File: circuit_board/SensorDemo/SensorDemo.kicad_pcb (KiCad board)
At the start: 4 copper layers, 65 x 57.5 mm, 56 parts, among them K1 PB, P1 CONN3X2, P2 CONN3X2, U1 TLV1117-33CDCYR, U2 dsPIC33EP32GP502, U3 LTC1658, U4 INA126, U5 REF1925, U6 REF1925, X1 CRYSTAL

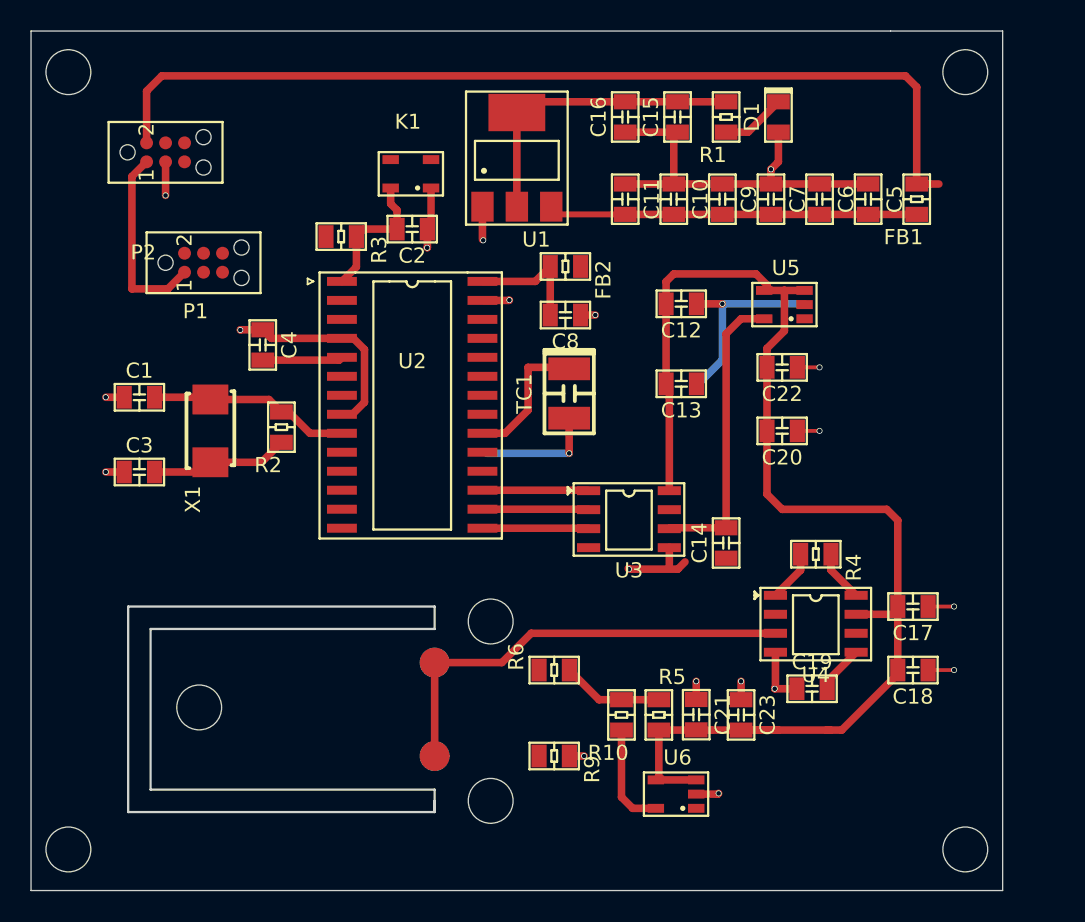
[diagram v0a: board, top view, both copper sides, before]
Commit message: PCB edited
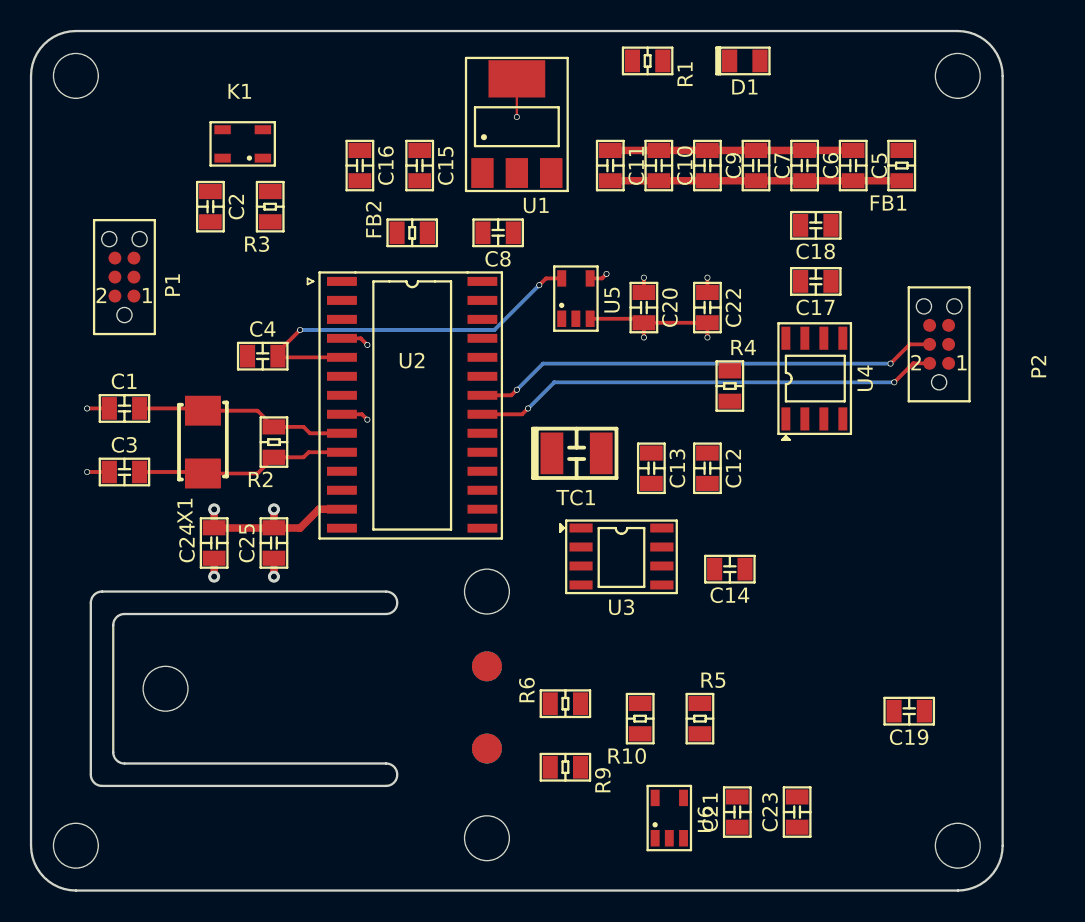
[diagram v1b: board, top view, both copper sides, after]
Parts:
- added C24: 1uF, SensorDemo_pcb:C0805, F.Cu at (129.8, 101.8)
- added C25: .1uF, SensorDemo_pcb:C0805, F.Cu at (133.8, 101.8)
- C1, C3: value C -> 22pF
- R10, R5: value 0 -> 0R
- R2: value R -> 1M
- TP1: moved to F.Cu
- TP3: moved to B.Cu
- X1: value CRYSTAL -> 8MHz
- moved P2 56.4 mm to (178.2, 91.0), turned to 90 degrees
- moved C18 30.5 mm to (170.0, 80.5)
- moved C17 22.7 mm to (170.0, 84.2)
- moved C16 18.0 mm to (139.5, 76.5), turned to 90 degrees
- moved C15 17.6 mm to (143.5, 76.5), turned to 90 degrees
- moved U5 16.2 mm to (153.0, 86.8), turned to 90 degrees
- moved U4 14.6 mm to (168.0, 90.8), turned to 90 degrees
- moved C2 13.6 mm to (129.5, 79.2), turned to 90 degrees
- moved R4 12.6 mm to (164.2, 91.2), turned to 90 degrees
- moved C20 12.4 mm to (158.5, 86.0), turned to 90 degrees
- moved K1 11.4 mm to (133.0, 76.0)
- moved C12 11.1 mm to (162.8, 96.8), turned to 90 degrees
- moved FB2 10.5 mm to (143.0, 81.0), turned to 180 degrees
- moved C23 7.50 mm to (168.8, 119.8), turned to 270 degrees
- moved C8 7.11 mm to (148.8, 81.0)
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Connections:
- C3 pad 1: Net-(C3-Pad1) -> /OSC2
- FB1 pad 1: /VDD -> Net-(FB1-Pad1)
- P1 pad 1: /~MCLR -> (no net)
- P1 pad 2: /VDD -> (no net)
- P2 pad 1: /~MCLR -> GND
- P2 pad 2: /VDD -> /ucTX
- P2 pad 4: /ucTX -> /ucRX
- P2 pad 5: (no net) -> Net-(FB1-Pad1)
- P2 pad 6: /ucRX -> Net-(FB1-Pad1)
- R2 pad 2: Net-(C3-Pad1) -> /OSC2
- U2 pad 10: /OSC1 -> /OSC2
- X1 pad 2: Net-(C3-Pad1) -> /OSC2
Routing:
- net +3V3: track 109.3 -> 24.1 mm, vias 0 -> 6
- net GND: track 96.6 -> 27.4 mm, vias 21 -> 8
- net /VDD: track 63.7 -> 0.00 mm
- net /ucRX: track 0.00 -> 31.3 mm, vias 0 -> 2
- net /ucTX: track 0.00 -> 31.3 mm, vias 0 -> 2
- net /Vsen: track 29.9 -> 0.00 mm
- net /OSC2: track 0.00 -> 13.9 mm
- net /~MCLR: track 12.9 -> 0.00 mm
- net Net-(TC1-Pad1): track 9.35 -> 0.00 mm
- net Net-(C3-Pad1): track 9.31 -> 0.00 mm
- net Net-(C2-Pad1): track 9.25 -> 0.00 mm
- net Net-(C8-Pad1): track 8.20 -> 0.00 mm
- net Net-(U2-Pad17): track 7.11 -> 0.00 mm
- net Net-(U2-Pad16): track 7.11 -> 0.00 mm
- net Net-(U2-Pad15): track 7.11 -> 0.00 mm
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- added copper zone on PWR, net +3V3
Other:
- outline, holes or cut-outs redrawn
